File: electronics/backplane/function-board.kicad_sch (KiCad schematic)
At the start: 4 parts, among them X3 MICROMOD_FUNCTION_BOARD_SOCKET

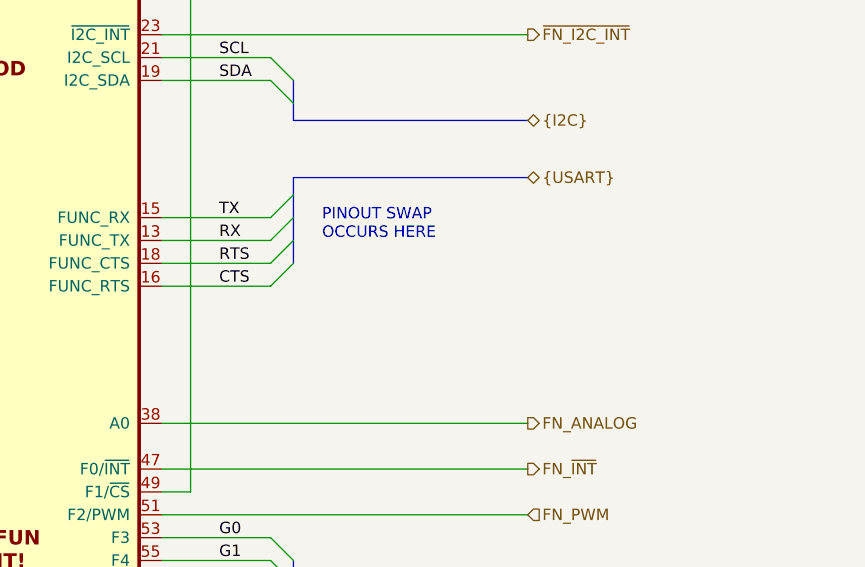
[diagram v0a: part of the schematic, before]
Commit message: Continue backplane
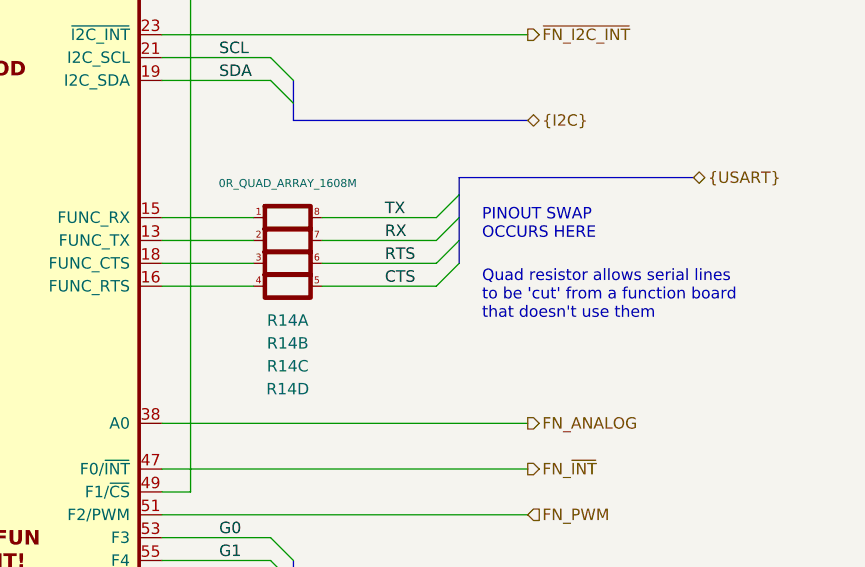
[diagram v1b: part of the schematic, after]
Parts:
- added R14: 0R_QUAD_ARRAY_1608M, Applidyne_Resistor:R_Array_Concave_4x1608M, symbol appli_resistor:0R_QUAD_ARRAY_1608M
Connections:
- net CTS: now also R14.5; no longer X3.16 (FUNC_RTS)
- net RTS: now also R14.6; no longer X3.18 (FUNC_CTS)
- net RX: now also R14.7; no longer X3.13 (FUNC_TX)
- net TX: now also R14.8; no longer X3.15 (FUNC_RX)
- new net: R14.3, X3.18 (FUNC_CTS)
- new net: R14.2, X3.13 (FUNC_TX)
- new net: R14.1, X3.15 (FUNC_RX)
- new net: R14.4, X3.16 (FUNC_RTS)
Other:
- note added: "Quad resistor allows serial lines to be 'cut' from a function board that doesn't use them"
